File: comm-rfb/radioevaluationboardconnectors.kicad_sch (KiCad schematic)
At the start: 4 parts, among them J2 TFM-110-02-SM-D-A-K-TR, J3 TFM-110-02-SM-D-A-K-TR

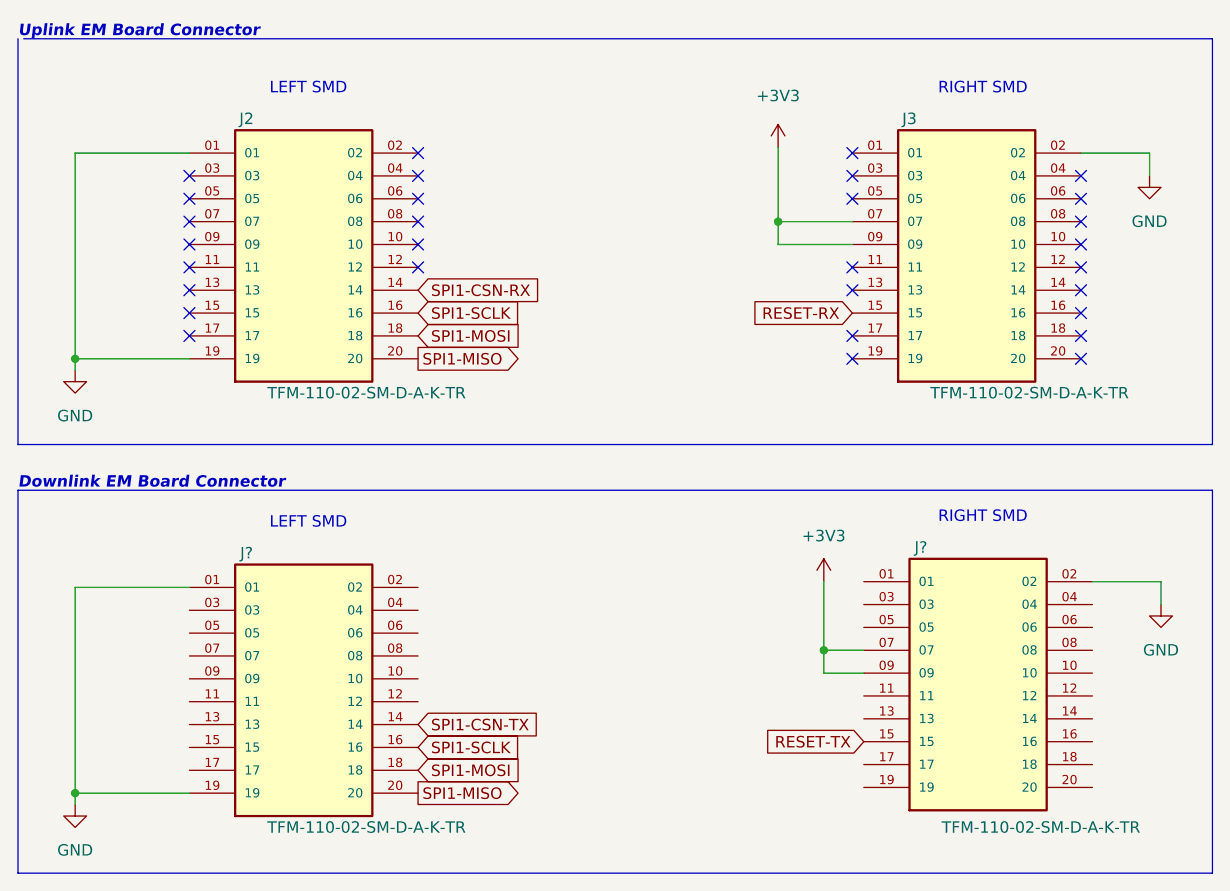
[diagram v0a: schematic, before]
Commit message: comm-rfb: reduce number of sheets in schematic
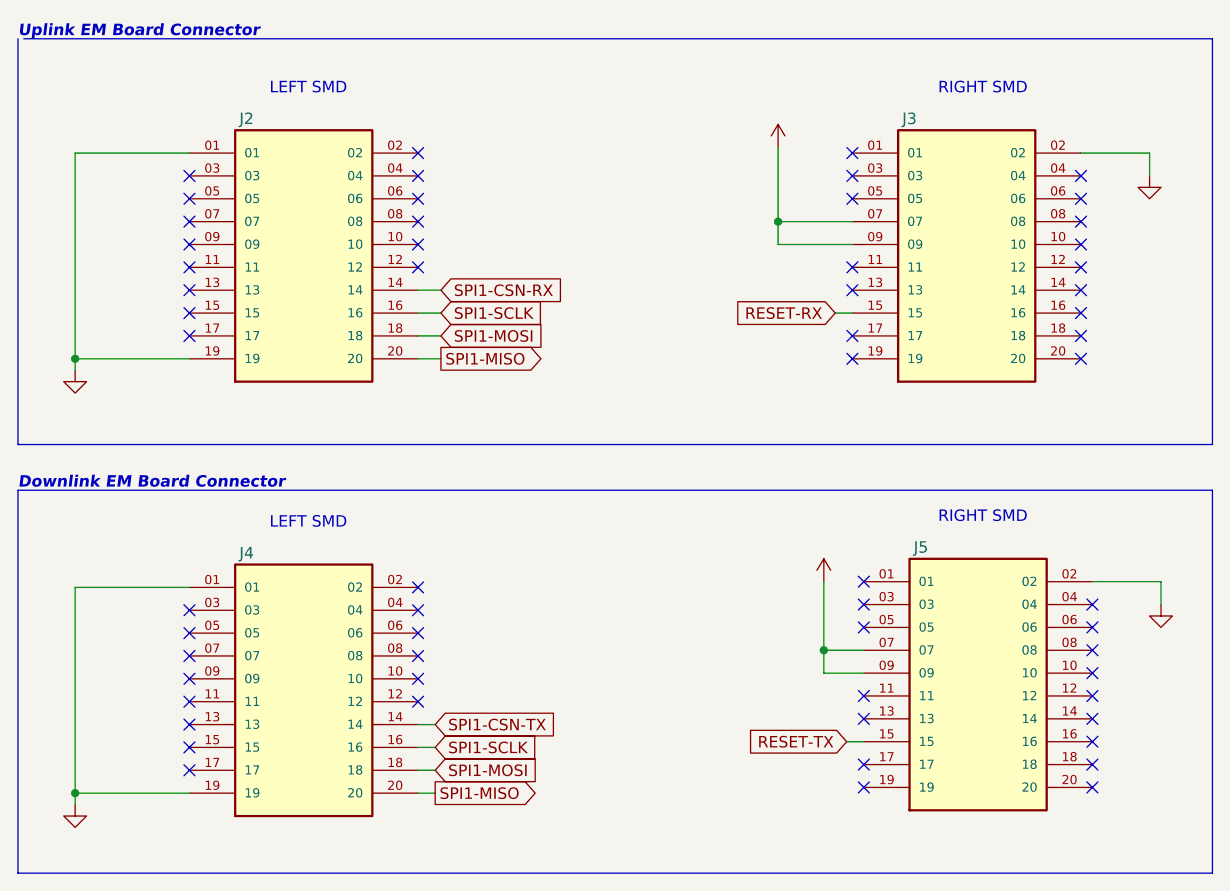
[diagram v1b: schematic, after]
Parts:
- J2, J3: value TFM-110-02-SM-D-A-K-TR -> (none); footprint SAMTEC_TFM-110-02-SM-D-A-K-TR -> (none)
- J4, J5: renamed from J?; value TFM-110-02-SM-D-A-K-TR -> (none); footprint SAMTEC_TFM-110-02-SM-D-A-K-TR -> (none)
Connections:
- no-connect marks 30 -> 60
